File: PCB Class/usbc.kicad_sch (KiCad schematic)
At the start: 3 parts, among them J1 USB_C_Receptacle_USB2.0

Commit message: Footprints
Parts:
- J1: footprint (none) -> Connector_USB:USB_C_Receptacle_GCT_USB4085
- R1, R2: footprint (none) -> Resistor_SMD:R_0603_1608Metric
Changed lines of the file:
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@@
     (property "Reference" "J1" (id 0) (at 129.54 60.96 0))
     (property "Value" "USB_C_Receptacle_USB2.0" (id 1) (at 129.54 63.5 0))
-    (property "Footprint" "" (id 2) (at 133.35 83.82 0)
+    (property "Footprint" "Connector_USB:USB_C_Receptacle_GCT_USB4085" (id 2) (at 133.35 83.82 0)
       (effects (font (size 1.27 1.27)) hide)
     )
@@
       (effects (font (size 1.27 1.27)) (justify left))
     )
-    (property "Footprint" "" (id 2) (at 156.972 81.28 90)
+    (property "Footprint" "Resistor_SMD:R_0603_1608Metric" (id 2) (at 156.972 81.28 90)
       (effects (font (size 1.27 1.27)) hide)
     )
@@
       (effects (font (size 1.27 1.27)) (justify left))
     )
-    (property "Footprint" "" (id 2) (at 167.132 80.01 90)
+    (property "Footprint" "Resistor_SMD:R_0603_1608Metric" (id 2) (at 167.132 80.01 90)
       (effects (font (size 1.27 1.27)) hide)
     )

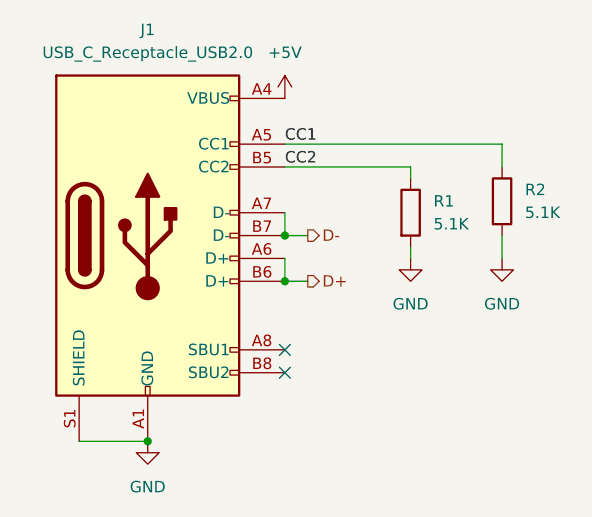
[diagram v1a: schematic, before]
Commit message: Final Layout
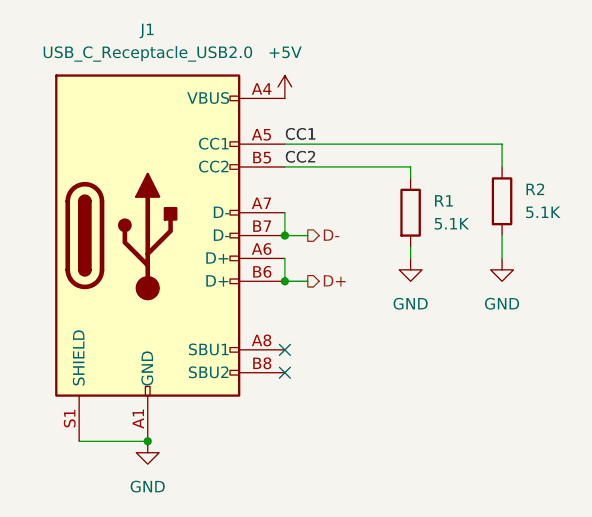
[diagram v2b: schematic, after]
